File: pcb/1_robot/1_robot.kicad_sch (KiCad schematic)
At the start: 0 parts

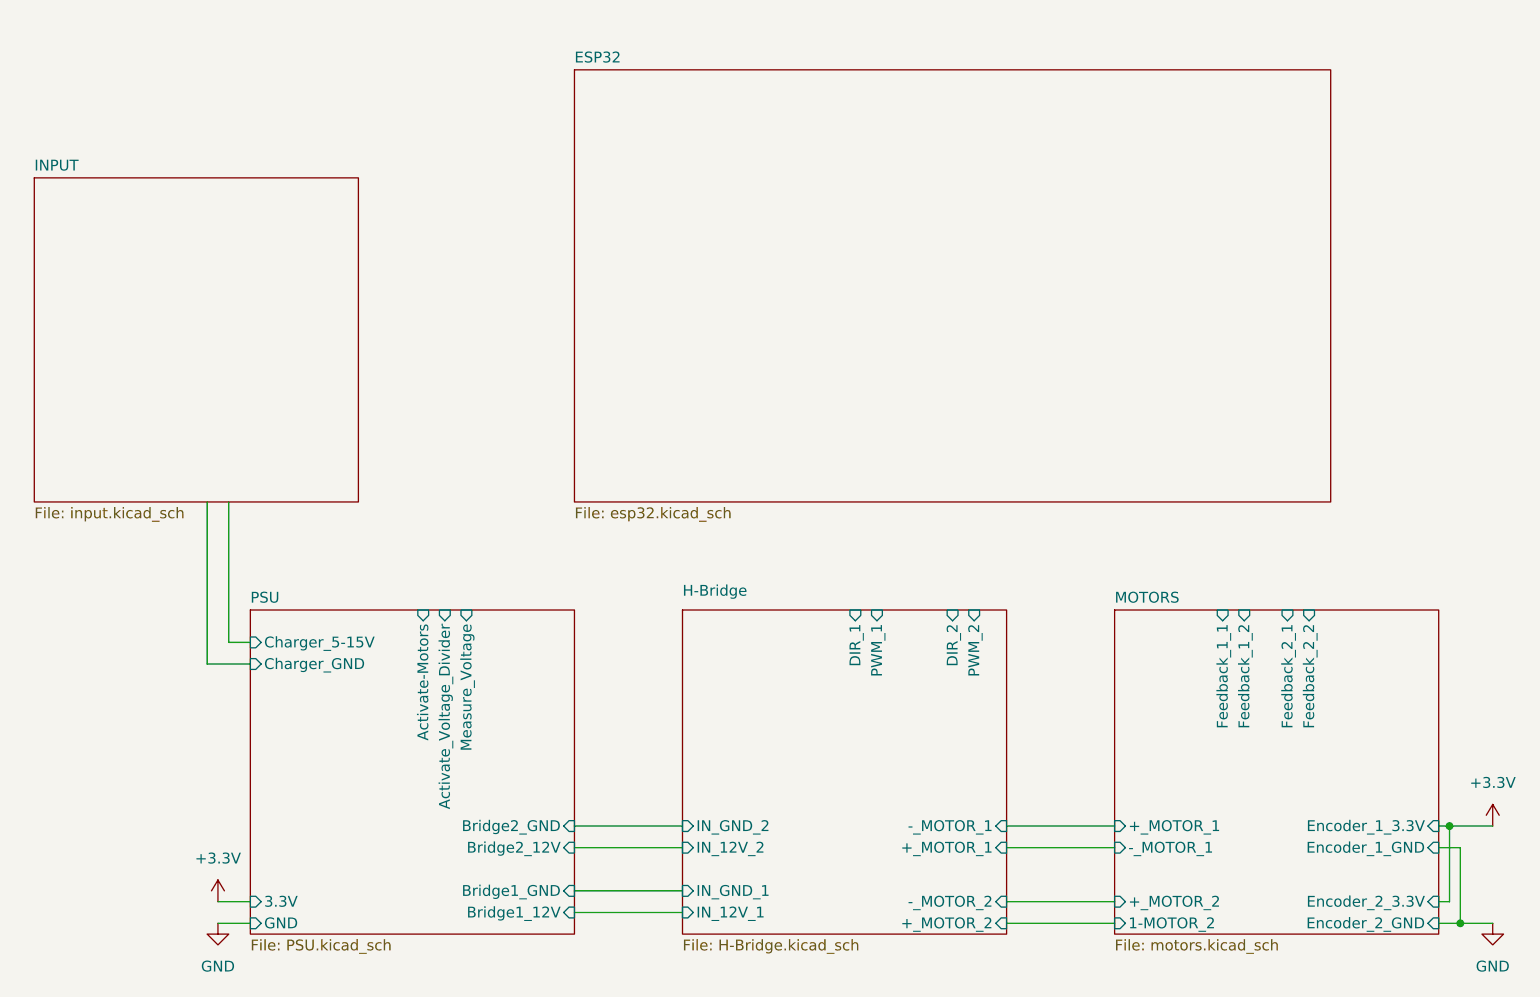
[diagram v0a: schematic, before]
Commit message: finished work
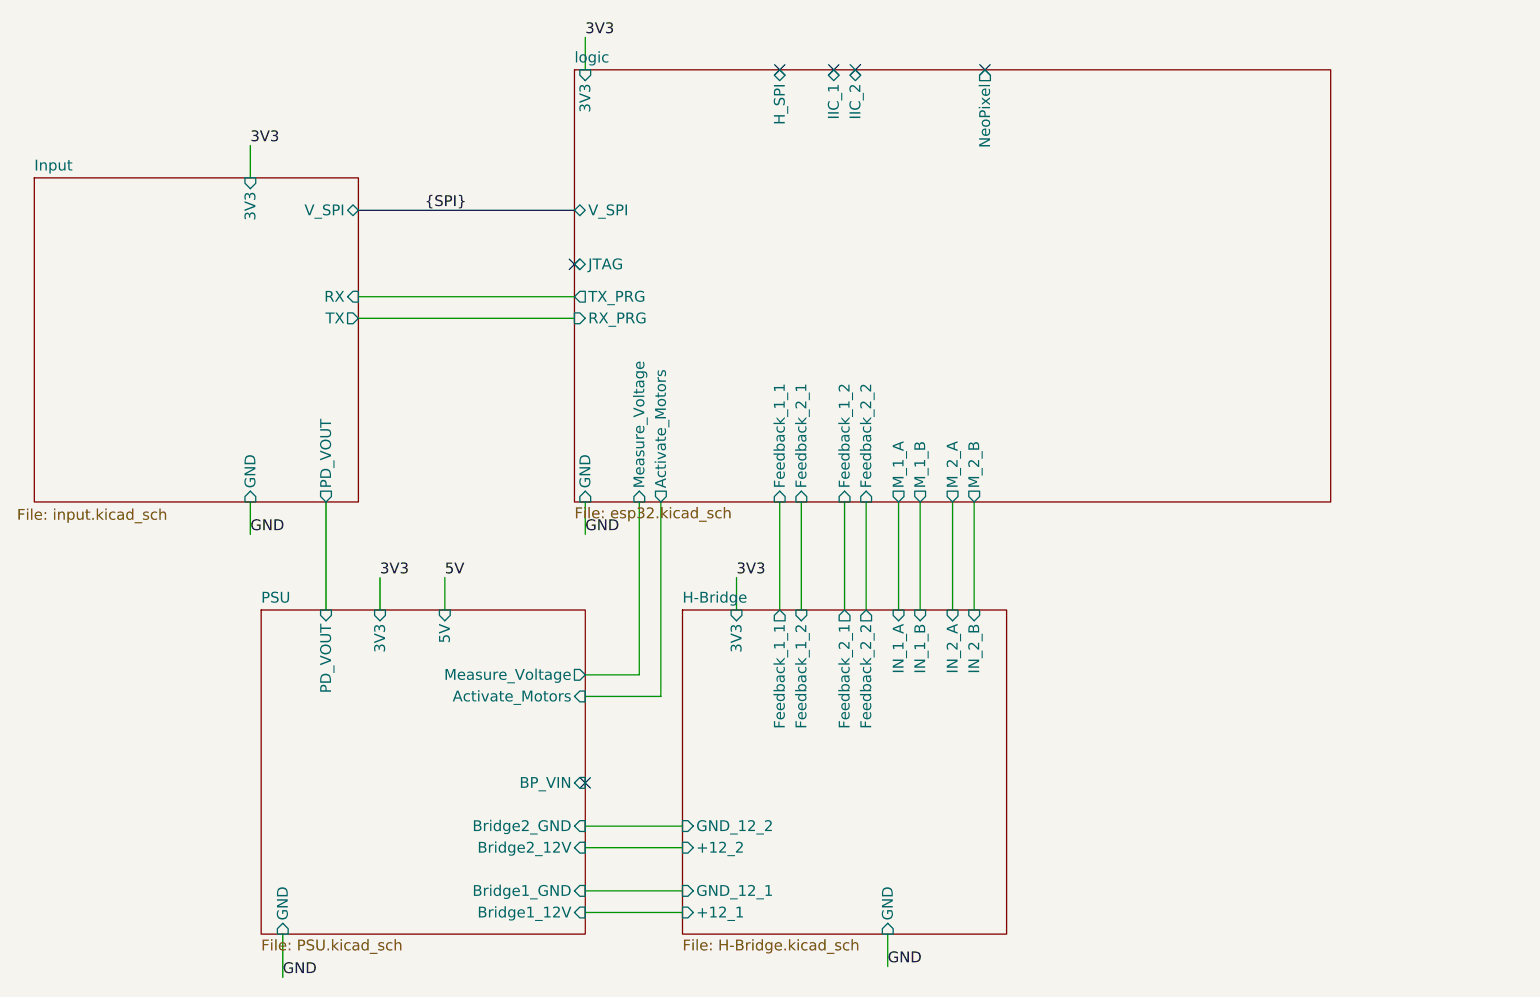
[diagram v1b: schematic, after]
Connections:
- no-connect marks 0 -> 6
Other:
- sheet ESP32 renamed logic
- sheet INPUT renamed Input
- removed sheet MOTORS
- sheet H-Bridge ports: added +12_1, +12_2, 3V3, Feedback_1_1, Feedback_1_2, Feedback_2_1, Feedback_2_2, GND, GND_12_1, GND_12_2, IN_1_A, IN_1_B, IN_2_A, IN_2_B; removed +_MOTOR_1, +_MOTOR_2, -_MOTOR_1, -_MOTOR_2, DIR_1, DIR_2, IN_12V_1, IN_12V_2, IN_GND_1, IN_GND_2, PWM_1, PWM_2
- sheet Input ports: added 3V3, GND, PD_VOUT, RX, TX, V_SPI; removed none
- sheet PSU ports: added 3V3, 5V, Activate_Motors, BP_VIN, PD_VOUT; removed 3.3V, Activate-Motors, Activate_Voltage_Divider, Charger_5-15V, Charger_GND
- sheet logic ports: added 3V3, Activate_Motors, Feedback_1_1, Feedback_1_2, Feedback_2_1, Feedback_2_2, GND, H_SPI, IIC_1, IIC_2, JTAG, M_1_A, M_1_B, M_2_A, M_2_B, Measure_Voltage, NeoPixel, RX_PRG, TX_PRG, V_SPI; removed none
